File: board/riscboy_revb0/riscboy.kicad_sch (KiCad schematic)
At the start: 74 parts

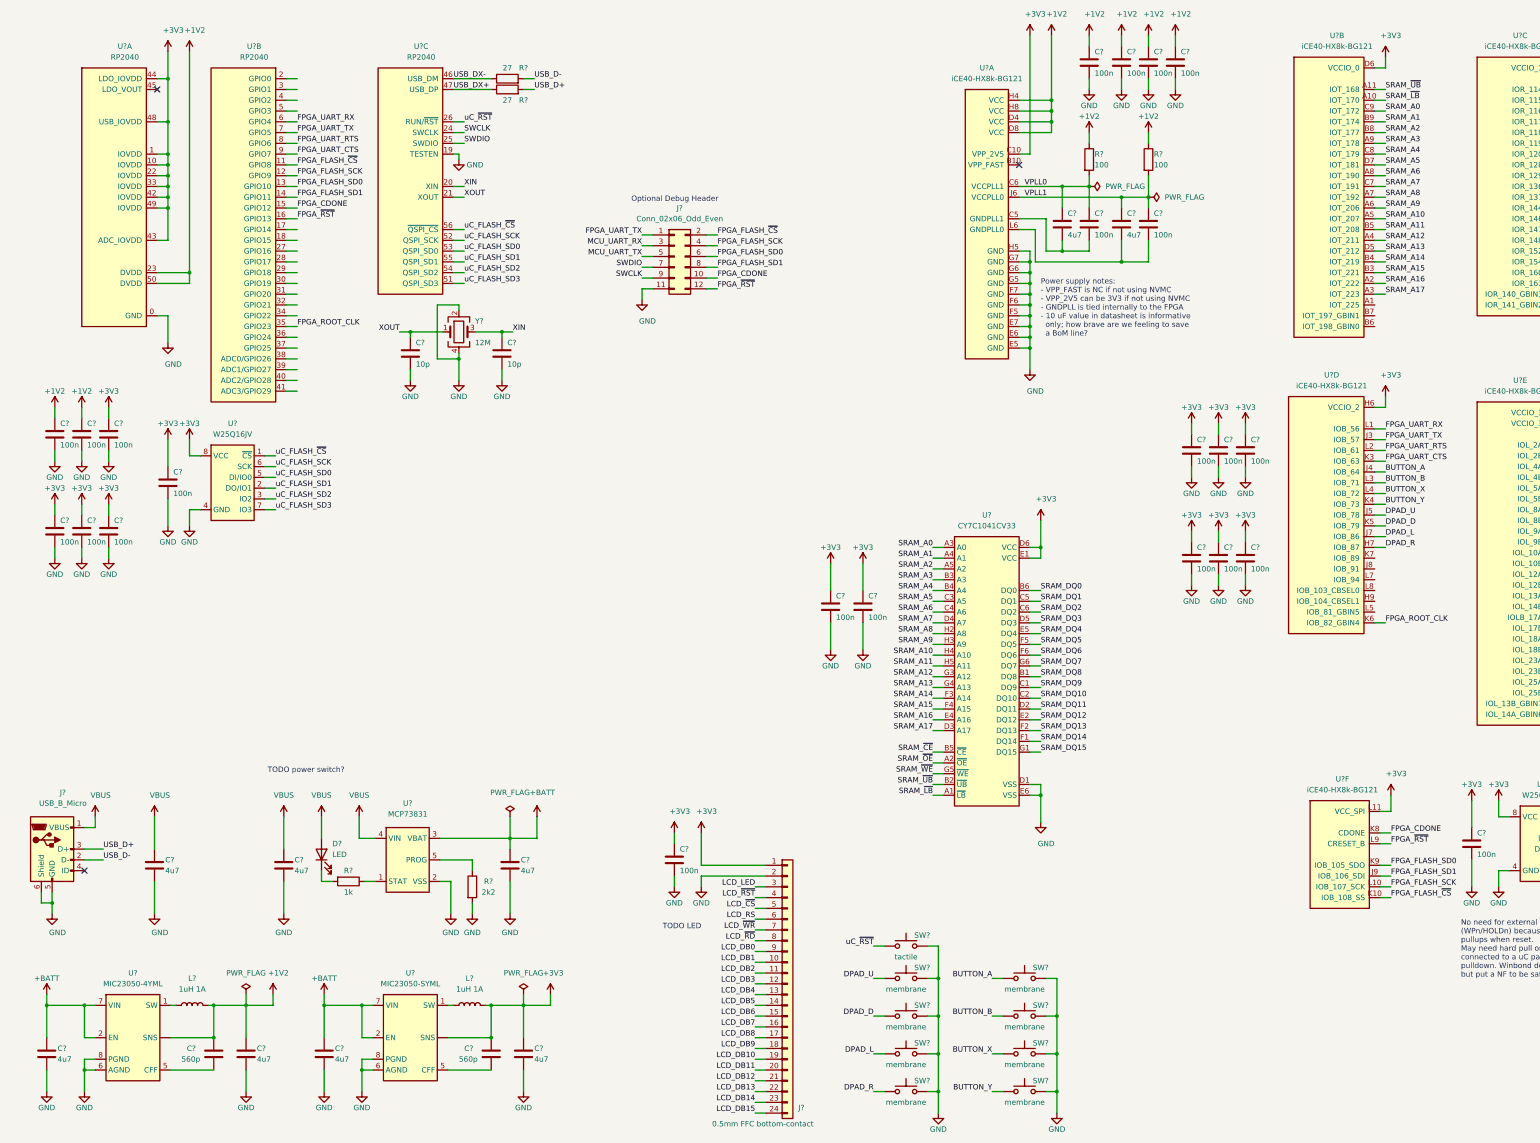
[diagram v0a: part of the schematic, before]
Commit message: More work on revb board schematic
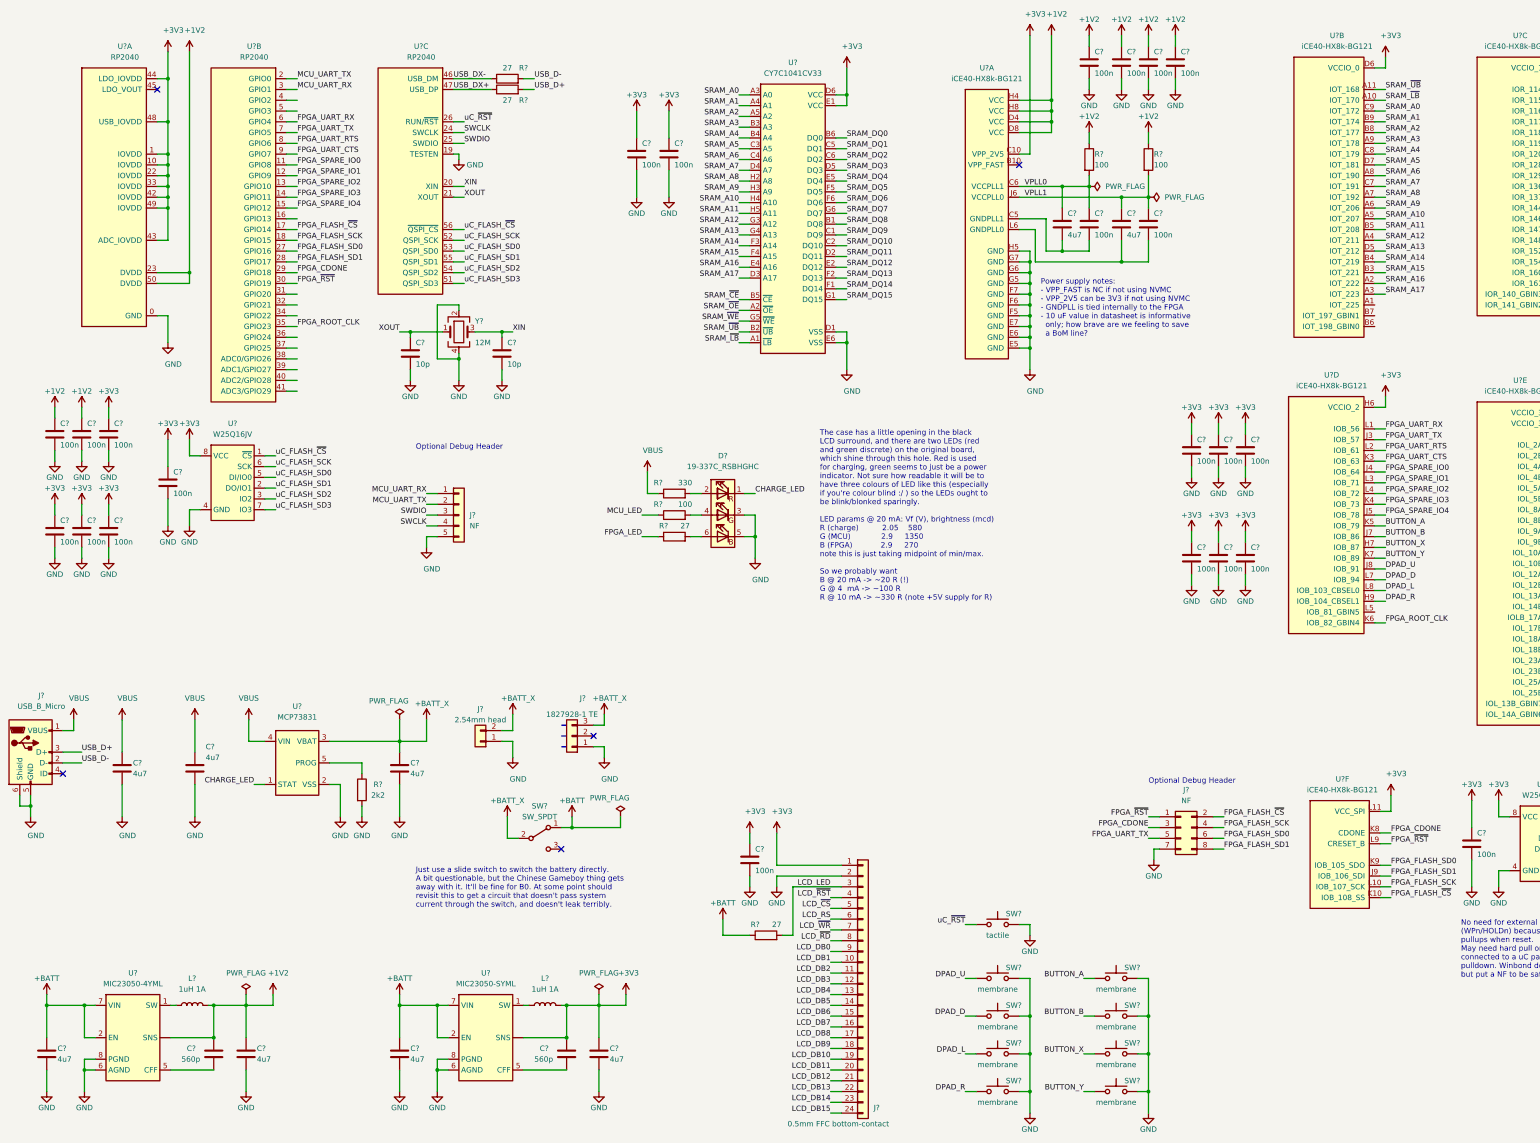
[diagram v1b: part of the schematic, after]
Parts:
- removed D?: LED, symbol Device:LED
- removed J?: Conn_02x06_Odd_Even, symbol Connector_Generic:Conn_02x06_Odd_Even
- removed R?: 1k, symbol Device:R
- added D?: 19-337C_RSBHGHC, symbol riscboy:LED_RGB_oddeven
- added J?: 1827928-1 TE, symbol Connector_Generic:Conn_01x03
- added J?: NF, symbol Connector_Generic:Conn_02x04_Odd_Even
- added J?: 2.54mm head, symbol Connector_Generic:Conn_01x02
- added J?: NF, symbol Connector_Generic:Conn_01x05
- added R? (x2): 27, symbol Device:R
- added R?: 330, symbol Device:R
- added R?: 100, symbol Device:R
- added SW?: SW_SPDT, symbol Switch:SW_SPDT
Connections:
- net +BATT: now also R?.1, SW?.1 (A); no longer C?.1, U?.3 (VBAT)
- net BUTTON_A: now also U?.K5 (IOB_79); no longer U?.J4 (IOB_64)
- net BUTTON_B: now also U?.J7 (IOB_86); no longer U?.L3 (IOB_71)
- net BUTTON_X: now also U?.H7 (IOB_87); no longer U?.L4 (IOB_72)
- net BUTTON_Y: now also U?.K7 (IOB_89); no longer U?.K4 (IOB_73)
- net DPAD_D: now also U?.L7 (IOB_94); no longer U?.K5 (IOB_79)
- net DPAD_L: now also U?.L8 (IOB_103_CBSEL0); no longer U?.J7 (IOB_86)
- net DPAD_R: now also U?.H9 (IOB_104_CBSEL1); no longer U?.H7 (IOB_87)
- net DPAD_U: now also U?.J8 (IOB_91); no longer U?.J5 (IOB_78)
- net FPGA_CDONE: now also U?.29 (GPIO18), J?.3 (Pin_3); no longer U?.15 (GPIO12)
- net FPGA_FLASH_SCK: now also U?.18 (GPIO15), J?.4 (Pin_4); no longer U?.12 (GPIO9)
- net FPGA_FLASH_SD0: now also U?.27 (GPIO16), J?.6 (Pin_6); no longer U?.13 (GPIO10)
- net FPGA_FLASH_SD1: now also U?.28 (GPIO17), J?.8 (Pin_8); no longer U?.14 (GPIO11)
- net FPGA_FLASH_~CS~: now also U?.17 (GPIO14), J?.2 (Pin_2); no longer U?.11 (GPIO8)
- net FPGA_UART_TX: now also J?.5 (Pin_5)
- net FPGA_~RST~: now also U?.30 (GPIO19), J?.1 (Pin_1); no longer U?.16 (GPIO13)
- net GND: now also D?.3 (GK), D?.5 (BK), J?.1 (Pin_1), J?.1 (Pin_1), J?.5 (Pin_5), J?.7 (Pin_7)
- net LCD_LED: now also R?.2
- net MCU_UART_RX: now also U?.3 (GPIO1), J?.1 (Pin_1)
- net MCU_UART_TX: now also U?.2 (GPIO0), J?.2 (Pin_2)
- net SWCLK: now also J?.4 (Pin_4)
- net SWDIO: now also J?.3 (Pin_3)
- net VBUS: now also R?.1
- net CHARGE_LED: now reaches U?.1 (STAT)
- net CHARGE_LED: now also D?.1 (RK)
- new net: D?.6 (BA), R?.2
- new net: D?.2 (RA), R?.2
- new net: D?.4 (GA), R?.2
- new net +BATT_X: C?.1, J?.2 (Pin_2), J?.3 (Pin_3), SW?.2 (B), U?.3 (VBAT)
- new net FPGA_LED: R?.1
- new net FPGA_SPARE_IO0: U?.11 (GPIO8), U?.J4 (IOB_64)
- new net FPGA_SPARE_IO1: U?.12 (GPIO9), U?.L3 (IOB_71)
- new net FPGA_SPARE_IO2: U?.13 (GPIO10), U?.L4 (IOB_72)
- new net FPGA_SPARE_IO3: U?.14 (GPIO11), U?.K4 (IOB_73)
- new net FPGA_SPARE_IO4: U?.15 (GPIO12), U?.J5 (IOB_78)
- new net MCU_LED: R?.1
- no-connect marks 3 -> 5
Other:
- note added: "Just use a slide switch to switch the battery directly. A bit questionable, but the Chinese Gameboy thing gets away with it. It'll be fine for B0. At some point should revisit this to get a circuit that doesn't pass system current through the switch, and doesn't leak terribly."
- note added: "The case has a little opening in the black LCD surround, and there are two LEDs (red and green discrete) on the original board, which shine through this hole. Red is used for charging, green seems to just be a power indicator. Not sure how readable it will be to have three colours of LED like this (especially if you're colour blind :/ ) so the LEDs ought to be blink/blonked sparingly. LED params 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"
- note removed: "TODO LED"
- note removed: "TODO power switch?"
- moved on the sheet: C?, J?, L?, R?, SW?, U?
